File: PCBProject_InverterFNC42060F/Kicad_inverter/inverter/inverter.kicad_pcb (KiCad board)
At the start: 4 copper layers, 100 x 106 mm, 103 parts, among them IC1 TLP2270_D4-LF4,E, IC2 TLP2270_D4-LF4,E, IC3 TLP2270_D4-LF4,E, J1 Conn_02x06_Top_Bottom, J10 Conn_01x06_Pin, J11 Header 2, J12 Conn_02x02_Odd_Even, J2 board_1, J3 board_1, J4 Conn_01x02_Pin, J5 Conn_01x02_Pin, J6 Header 2, J7 Header 2, J8 Header 2, J9 Header 2, Q1 FMMT618TA, Q2 FNC42060F, U1 VIPER22A, U2 LM2675M-5.0

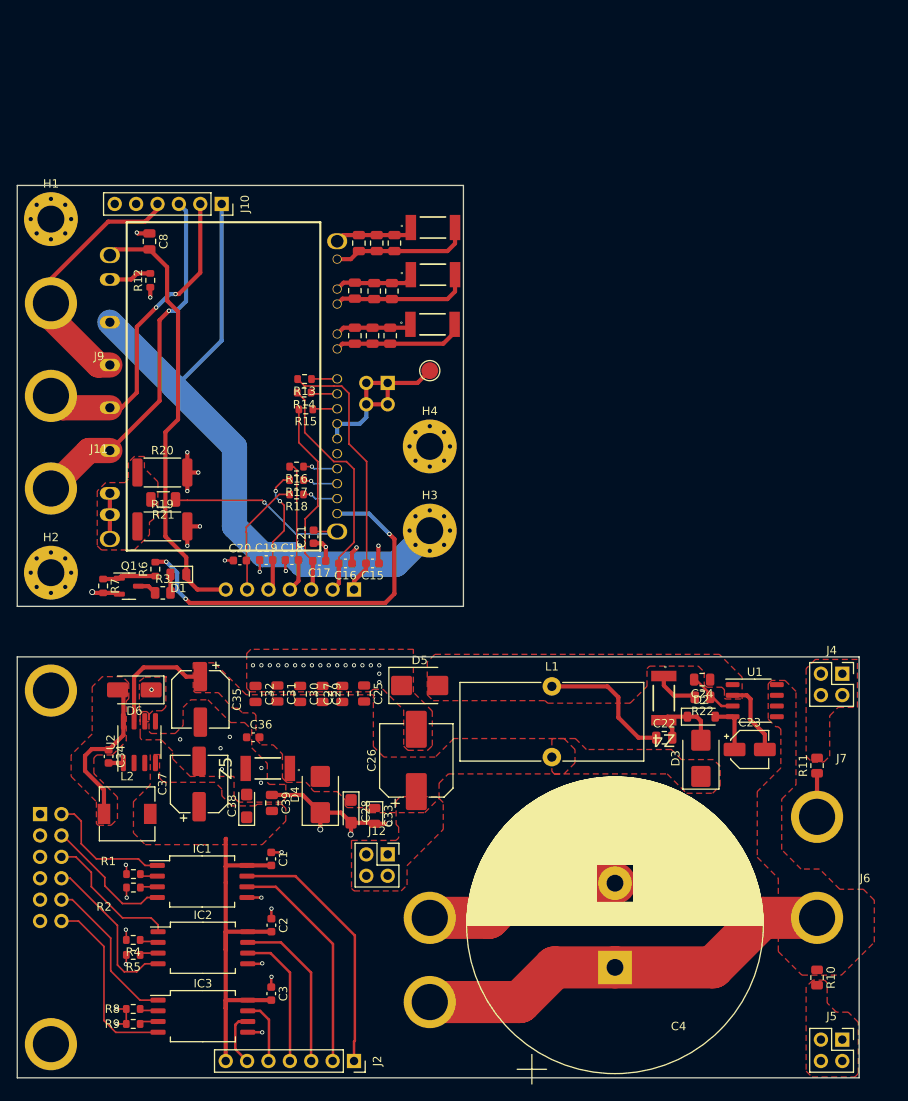
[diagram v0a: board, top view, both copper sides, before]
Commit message: update inverter board
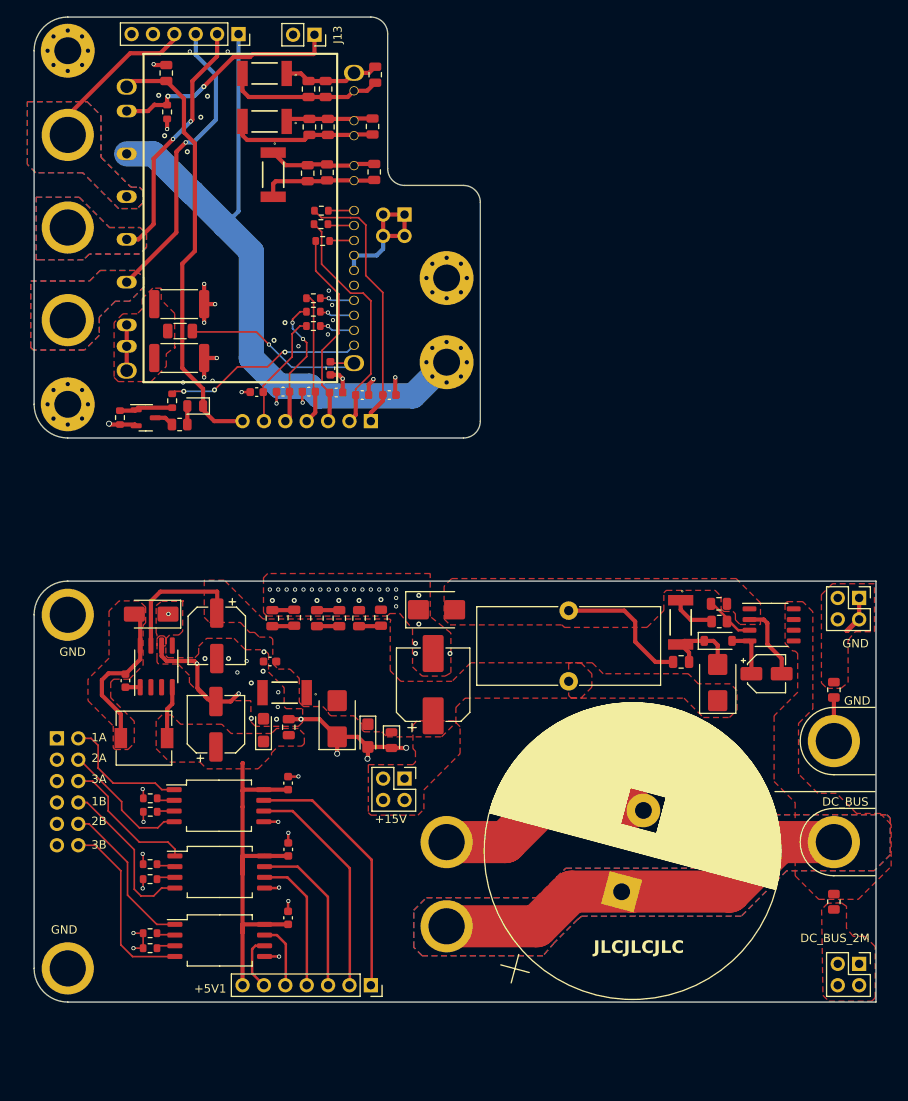
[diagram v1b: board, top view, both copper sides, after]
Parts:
- removed the ? at (23.0, 109.0)
- removed the ? at (68.0, 136.0)
- removed the ? at (23.0, 151.0)
- removed the ? at (68.0, 146.0)
- removed the J12 at (63.0, 128.5)
- removed the J12 at (63.0, 72.5)
- removed TP7: TP-黄色测试点, TestPoint:TestPoint_Pad_D2.0mm
- added ?: , , F.Cu at (70.0, 127.0)
- added ?: , , F.Cu at (25.0, 142.0)
- added ?: , , F.Cu at (25.0, 100.0)
- added ?: , , F.Cu at (70.0, 137.0)
- added J12: Conn_02x02_Odd_Even, Connector_PinSocket_2.54mm:PinSocket_2x02_P2.54mm_Vertical, F.Cu at (65.0, 119.5)
- added J12: Conn_02x02_Odd_Even, Connector_PinSocket_2.54mm:PinSocket_2x02_P2.54mm_Vertical, B.Cu at (65.0, 52.5)
- added J13: Conn_01x02_Pin, Connector_PinSocket_2.54mm:PinSocket_1x02_P2.54mm_Vertical, F.Cu at (54.3, 31.1)
- moved Z1 27.1 mm to (48.4, 35.7), turned to 180 degrees
- moved Z2 27.0 mm to (48.4, 41.4), turned to 180 degrees
- moved Z3 26.0 mm to (49.4, 47.7), turned to -90 degrees
- moved C9 21.0 mm to (53.7, 42.0)
- moved C11 20.9 mm to (55.9, 42.0)
- moved C12 20.8 mm to (55.8, 47.5)
- moved C13 20.8 mm to (53.5, 47.5)
- moved J10 20.3 mm to (45.3, 31.0)
- moved R16 20.1 mm to (54.2, 62.4)
- moved C15 20.1 mm to (63.2, 73.9)
- moved C16 20.1 mm to (60.0, 73.9)
- moved C17 20.1 mm to (56.9, 73.6)
- moved C18 20.1 mm to (53.6, 73.5)
- moved C19 20.1 mm to (50.6, 73.5)
- moved C20 20.1 mm to (47.4, 73.5)
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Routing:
- net /TEMP1: track 5.14 -> 27.9 mm, vias 0 -> 2
- net /DSP_PWM1_~{FAULT_5V}: track 46.7 -> 24.0 mm
- net GND: track 111.3 -> 131.5 mm, vias 48 -> 83
- net /U: track 30.7 -> 19.5 mm
- net /V: track 37.7 -> 29.5 mm
- net /W: track 42.8 -> 35.2 mm
- net /GND_2M: track 0.00 -> 6.58 mm
- net +5V1: track 98.2 -> 104.5 mm
- net +15V1: track 36.9 -> 40.8 mm
- net /M+3: track 9.18 -> 12.8 mm
- net /M-1: track 16.7 -> 18.8 mm
- net /M+1: track 9.63 -> 11.6 mm
- net /M-3: track 15.7 -> 13.8 mm
- net DC_BUS: track 131.3 -> 132.5 mm
- net /M-2: track 16.7 -> 17.7 mm
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- added copper zone on B.Cu, net /U
- added copper zone on F.Cu, net /U
- added copper zone on In1.Cu, net /U
- added copper zone on In2.Cu, net /U
- added copper zone on B.Cu, net /V
- added copper zone on F.Cu, net /V
- added copper zone on In1.Cu, net /V
- added copper zone on In2.Cu, net /V
- added copper zone on B.Cu, net /W
- added copper zone on F.Cu, net /W
- added copper zone on In1.Cu, net /W
- added copper zone on In2.Cu, net /W
- added copper zone on B.Cu, net DC_BUS
- added copper zone on In1.Cu, net DC_BUS
- added copper zone on In2.Cu, net DC_BUS
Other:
- board size 100 x 106 mm -> 100 x 117 mm
- board text added: "+15V"
- board text added: "+5V1"
- board text added: "1A"
- board text added: "1B"
- board text added: "2A"
- board text added: "2B"
- board text added: "3A"
- board text added: "3B"
- board text added: "DC_BUS"
- board text added: "DC_BUS_2M"
- board text added: "GND"
- board text added: "JLCJLCJLC"
- board text added: "inverter test board part 1 2023/12/13"
